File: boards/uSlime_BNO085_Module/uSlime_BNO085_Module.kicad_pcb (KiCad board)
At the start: 2 copper layers, 16.8 x 15.5 mm, 15 parts, among them J1 Conn_01x05, U1 BNO085

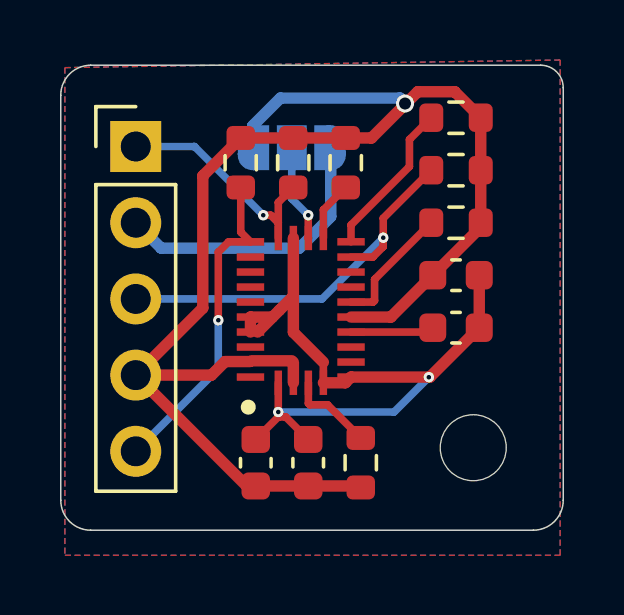
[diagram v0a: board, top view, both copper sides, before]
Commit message: gerber update
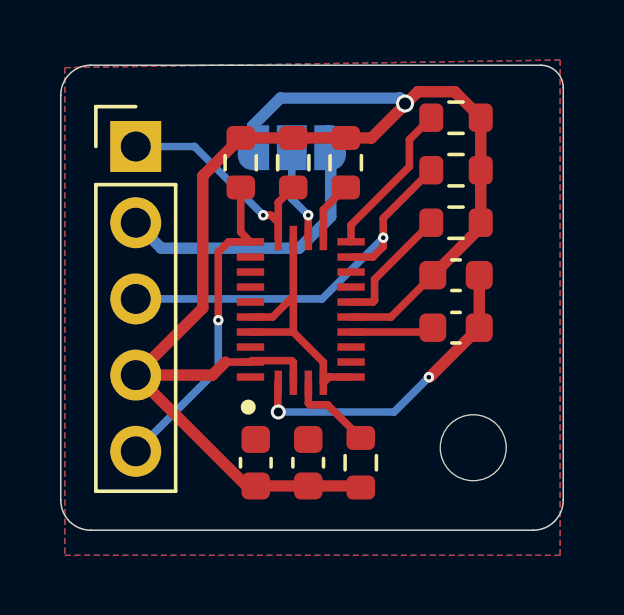
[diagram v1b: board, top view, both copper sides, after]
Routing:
- net GND: track 35.0 -> 29.6 mm
